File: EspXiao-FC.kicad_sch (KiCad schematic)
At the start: 11 parts, among them J1 Conn_01x08_Pin, J2 Conn_01x02_Pin, J3 Conn_01x02_Pin, J4 Conn_01x02_Pin, J5 Conn_01x02_Pin, J6 Conn_01x02_Pin, Q1 IRFZ44N, Q2 IRFZ44N, Q3 IRFZ44N, Q4 IRFZ44N, U1 MOUDLE-SEEEDUINO-XIAO-ESP32S3

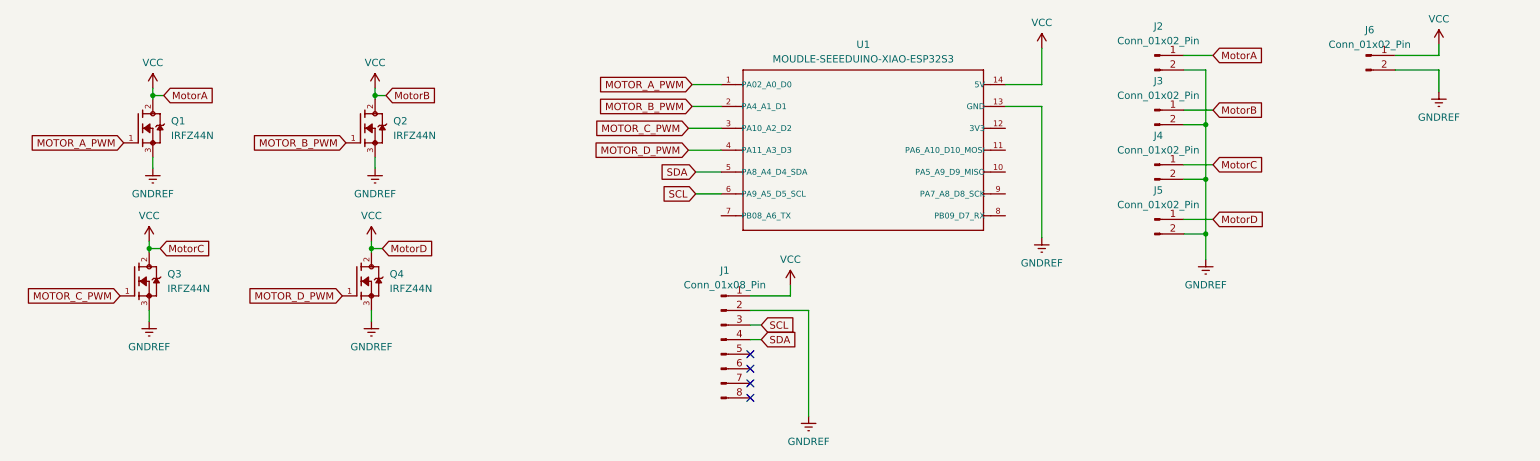
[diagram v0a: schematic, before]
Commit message: Complete
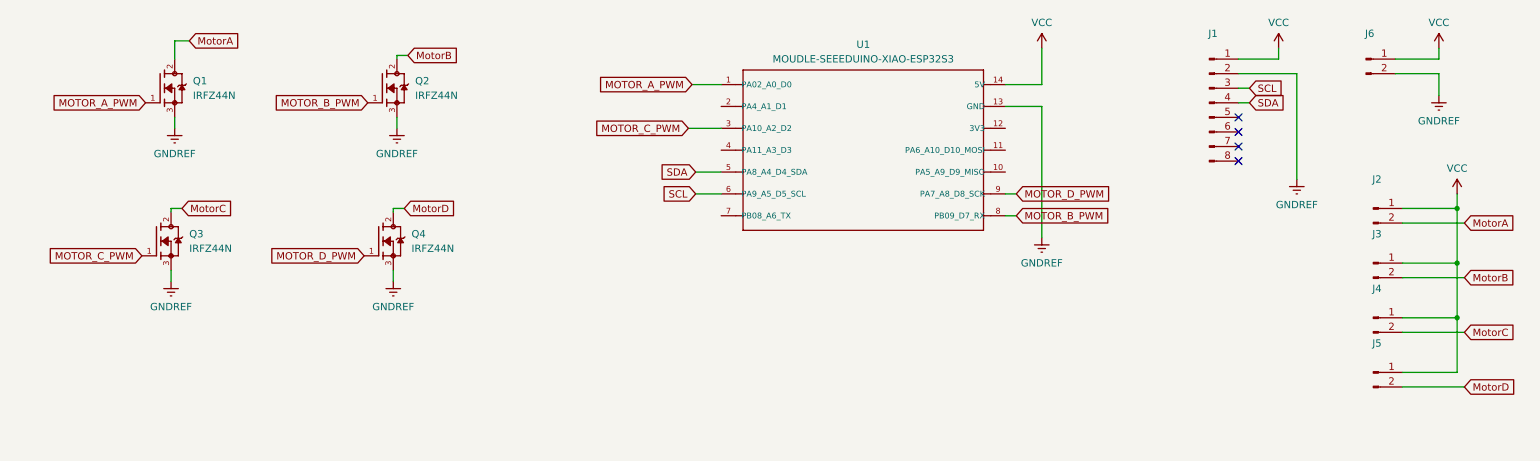
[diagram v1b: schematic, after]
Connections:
- net GNDREF: no longer J2.2 (Pin_2), J3.2 (Pin_2), J4.2 (Pin_2), J5.2 (Pin_2)
- net MOTOR_B_PWM: now also U1.8 (PB09_D7_RX); no longer U1.2 (PA4_A1_D1)
- net MOTOR_D_PWM: now also U1.9 (PA7_A8_D8_SCK); no longer U1.4 (PA11_A3_D3)
- net VCC: no longer Q1.2, Q2.2, Q3.2, Q4.2
- new net MotorA: J2.2 (Pin_2), Q1.2
- new net MotorB: J3.2 (Pin_2), Q2.2
- new net MotorC: J4.2 (Pin_2), Q3.2
- new net MotorD: J5.2 (Pin_2), Q4.2
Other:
- moved on the sheet: J1, J2, J3, J4, J5, J6, Q1, Q2, Q3, Q4
